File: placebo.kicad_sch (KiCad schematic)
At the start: 12 parts

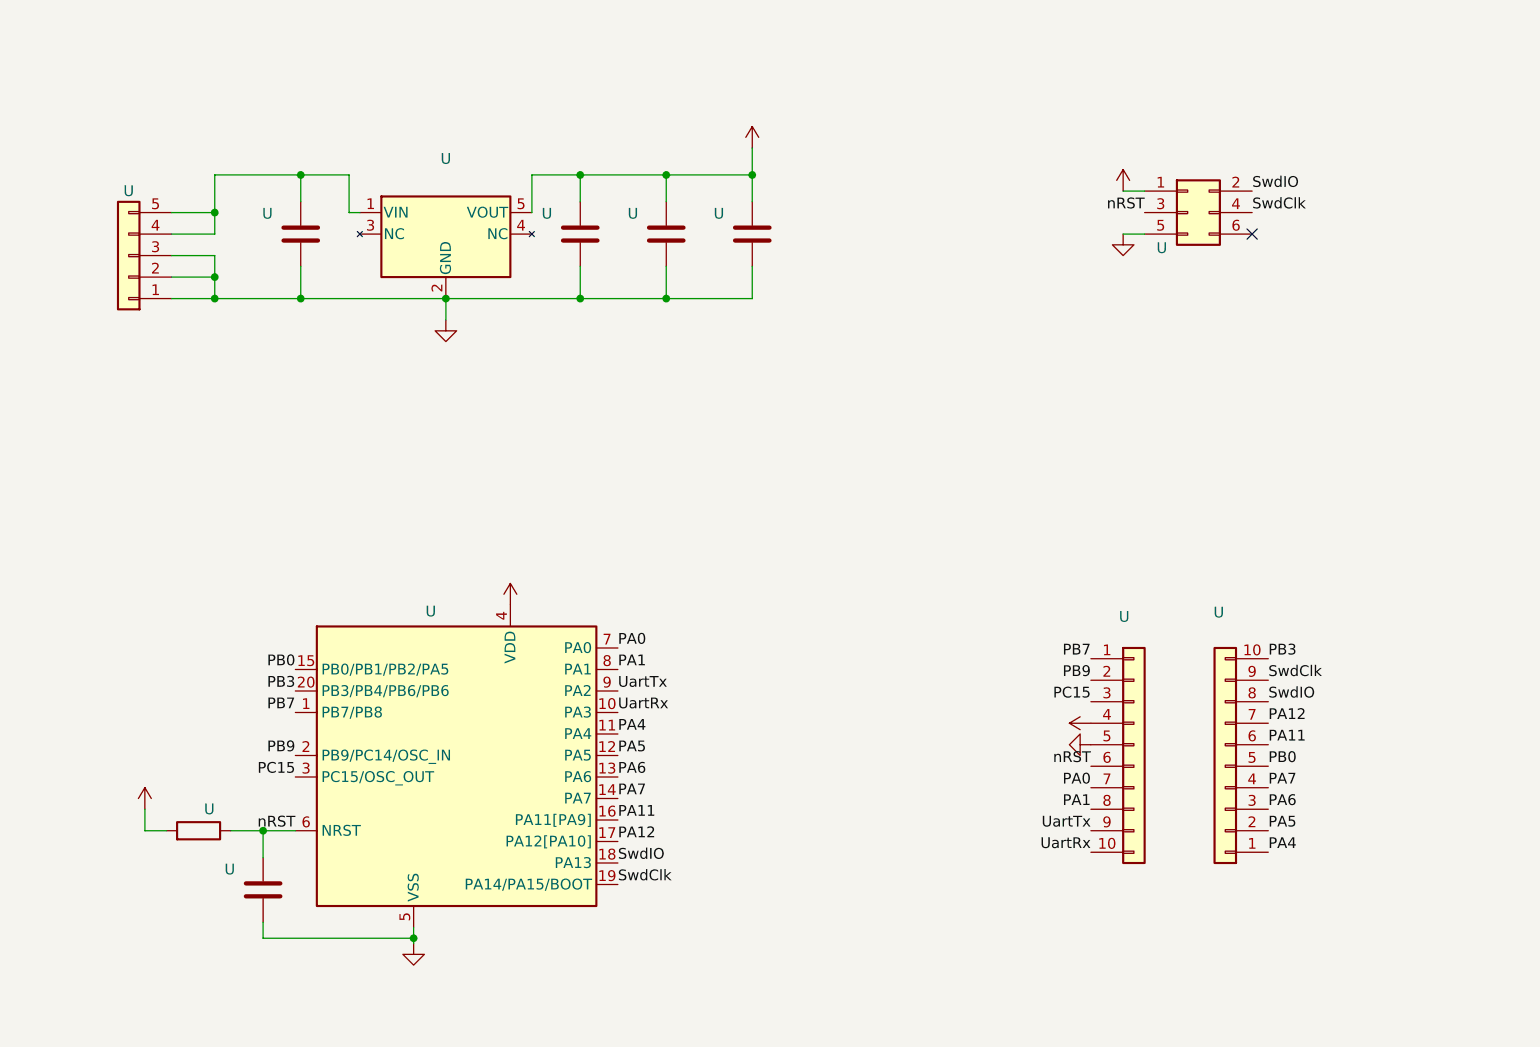
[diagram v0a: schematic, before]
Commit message: PlaceboConnect
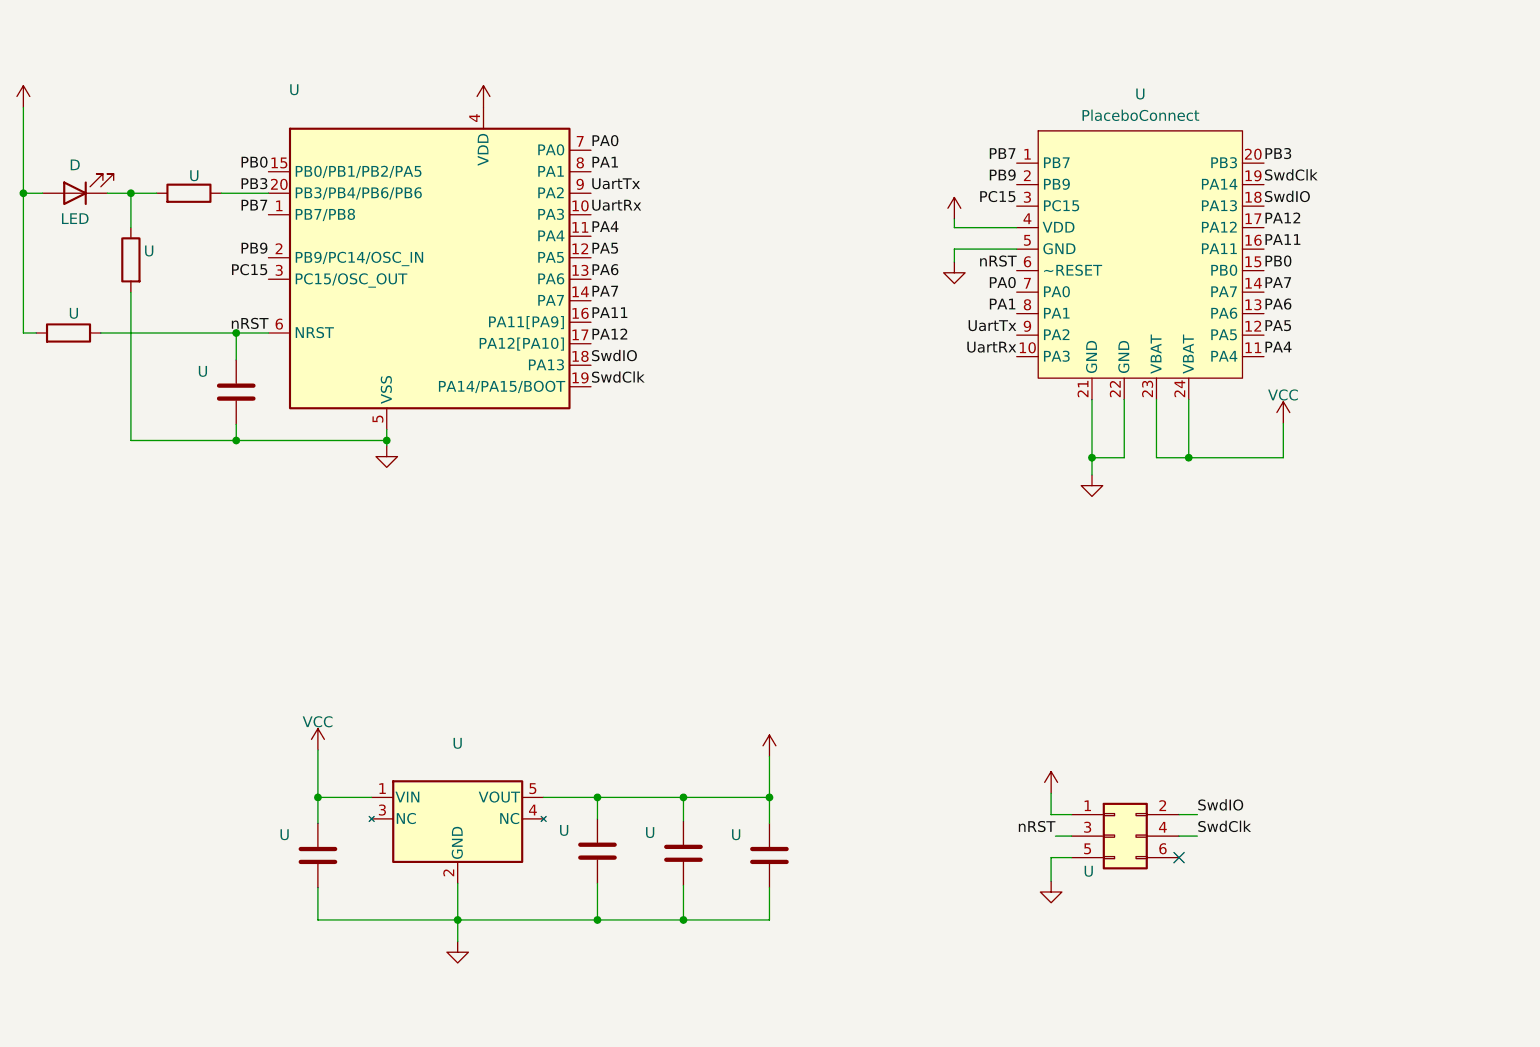
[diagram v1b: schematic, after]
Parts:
- removed U (x2): (no value), symbol Connector_Generic:Conn_01x10
- removed U: (no value), symbol Connector_Generic:Conn_01x05
- added D: LED, symbol Device:LED
- added U (x2): (no value), symbol Device:R
- added U: PlaceboConnect, placebo:PlaceboConnect, symbol Placebo:PlaceboConnect
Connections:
- net +3V3: now also D.2 (A), U.4 (VDD)
- net GND: now also U.2, U.21 (GND), U.22 (GND), U.5 (GND)
- net PA0: now also U.7 (PA0)
- net PA1: now also U.8 (PA1)
- net PA11: now also U.16 (PA11)
- net PA12: now also U.17 (PA12)
- net PA4: now also U.11 (PA4)
- net PA5: now also U.12 (PA5)
- net PA6: now also U.13 (PA6)
- net PA7: now also U.14 (PA7)
- net PB0: now also U.15 (PB0)
- net PB3: now also U.1, U.20 (PB3)
- net PB7: now also U.1 (PB7)
- net PB9: now also U.2 (PB9)
- net PC15: now also U.3 (PC15)
- net SwdClk: now also U.19 (PA14)
- net SwdIO: now also U.18 (PA13)
- net UartRx: now also U.10 (PA3)
- net UartTx: now also U.9 (PA2)
- net nRST: now also U.6 (~RESET)
- net VCC: now reaches U.1, U.1 (VIN)
- net VCC: now also U.23 (VBAT), U.24 (VBAT)
- new net: D.1 (K), U.1, U.2
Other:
- moved on the sheet: U

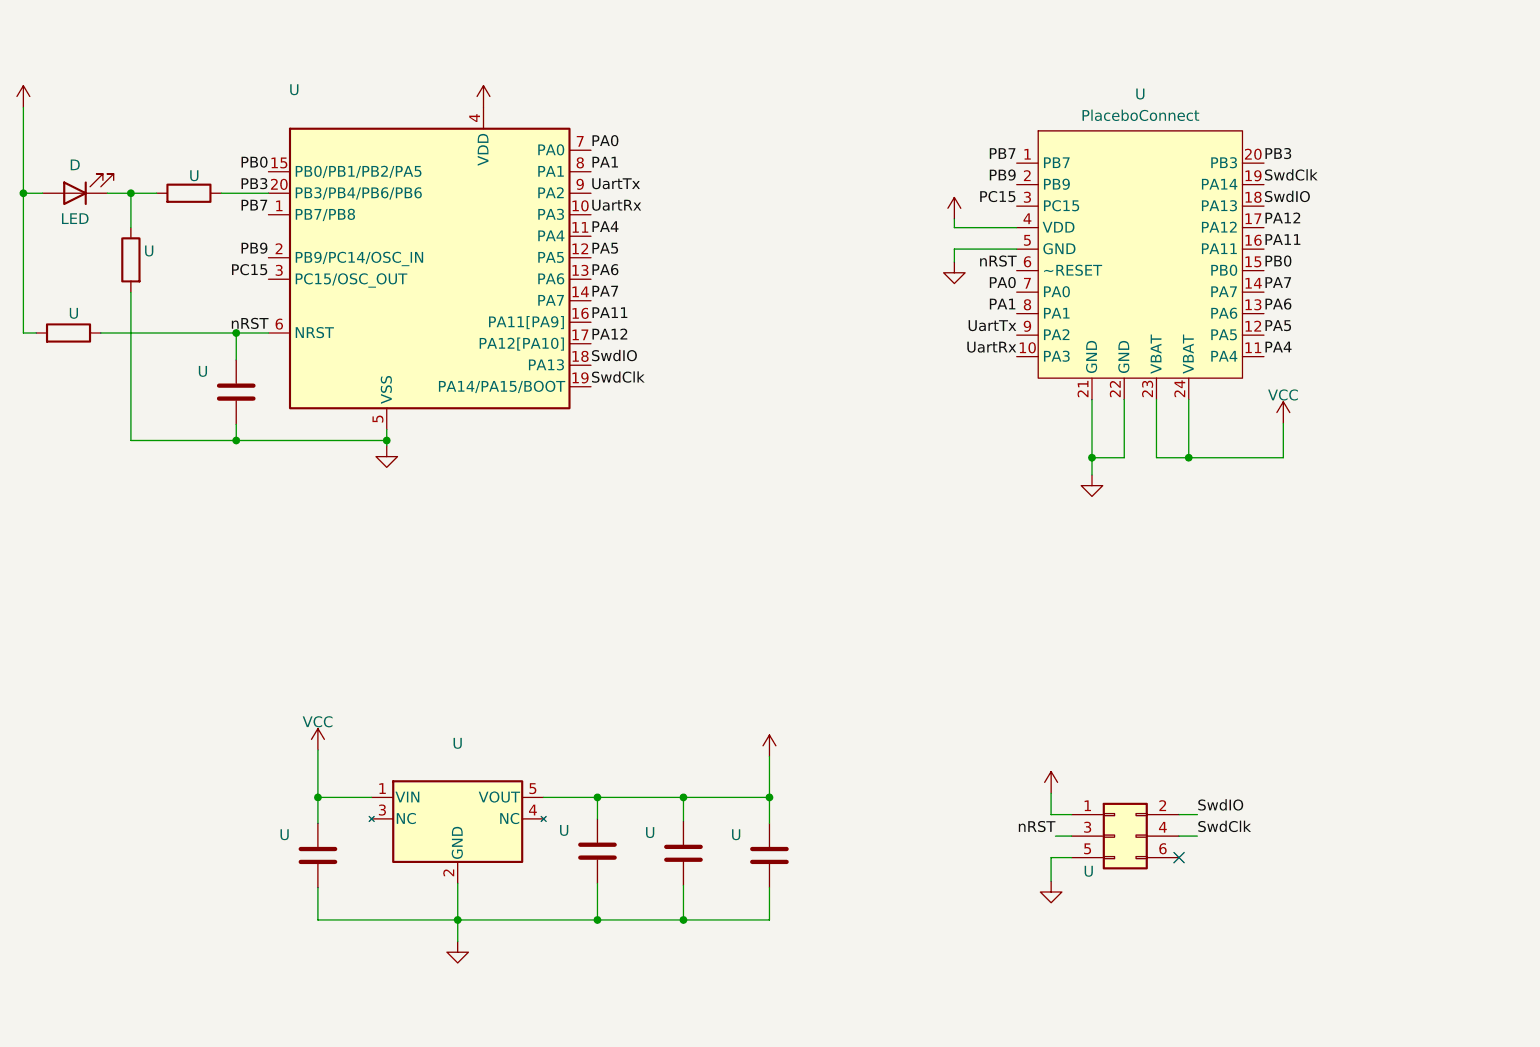
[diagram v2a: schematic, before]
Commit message: rev. 0x6
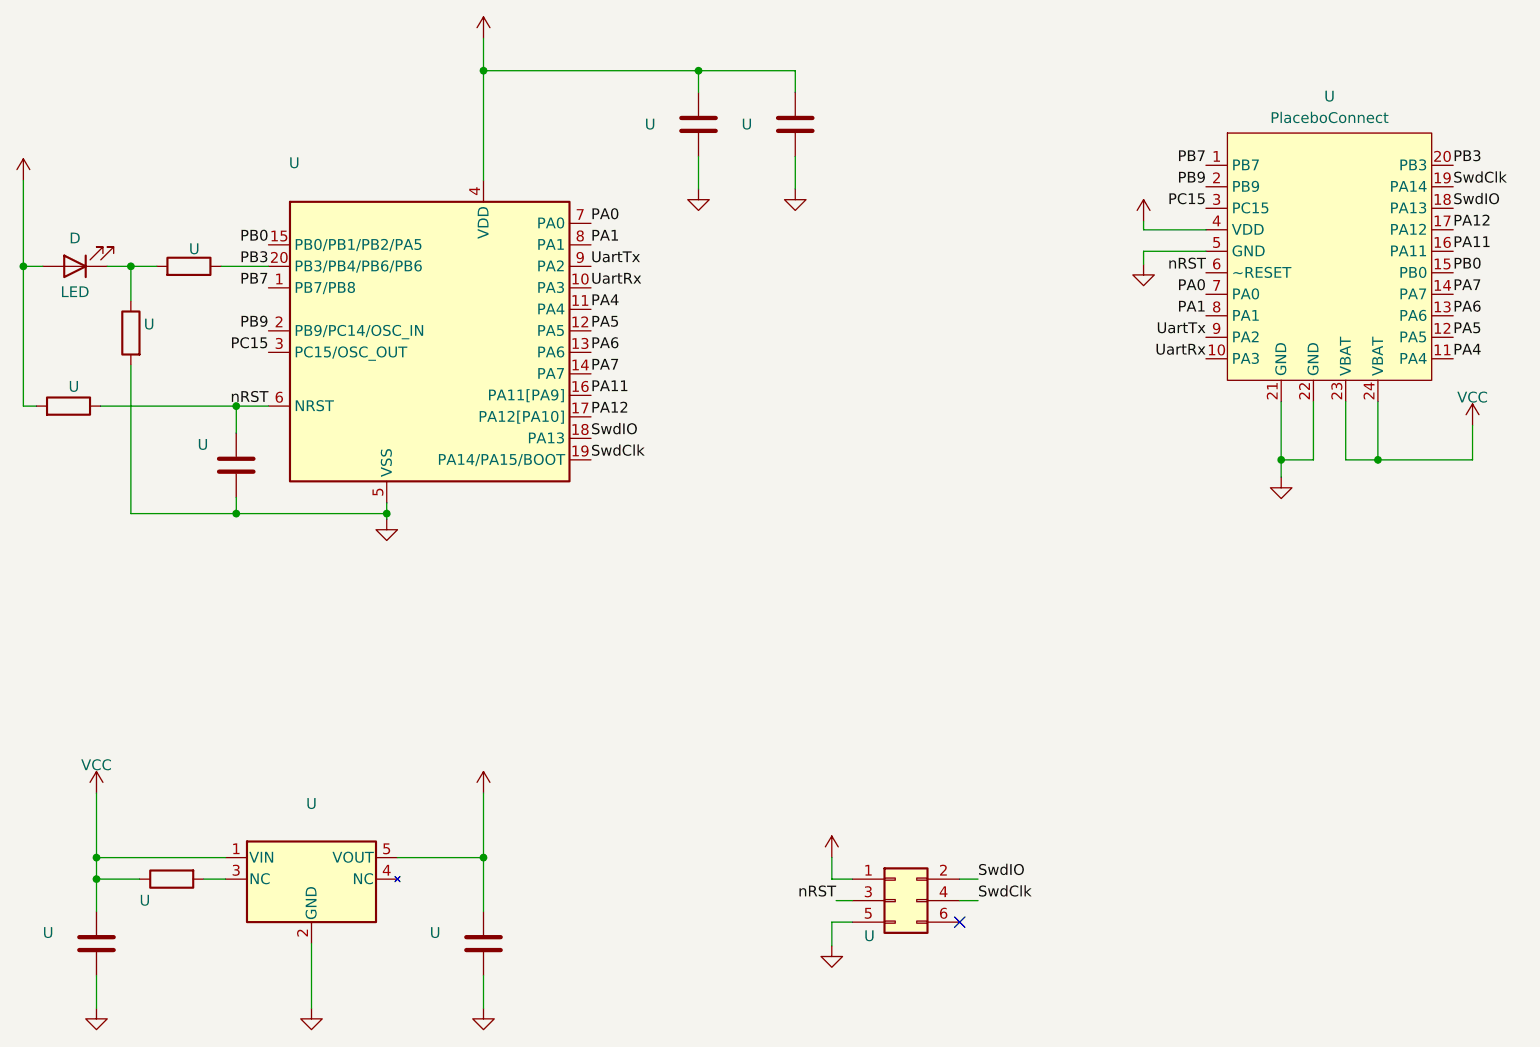
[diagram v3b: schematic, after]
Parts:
- added U: (no value), symbol Device:R
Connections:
- net VCC: now also U.1
- net at U.3 (NC): now also U.2
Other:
- moved on the sheet: D, U
